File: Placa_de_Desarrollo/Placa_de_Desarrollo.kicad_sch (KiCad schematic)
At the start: 46 parts, among them J10 5V_OUT, J11 3.3V_OUT, J12 ADC_VREF, J13 GND, J14 AGND, J15 VSYS_ALIMEANTACION_EXTERNA, J16 3V3_EN, J17 DEVICE I2C0, J18 PINES GPIO, J19 ADC1, J2 USB_B_Micro, J20 ADC2, J21 ADC0, J3 DEVICE I2C0, J4 GND, J5 GND, J6 GND, J7 GND, J8 GND, J9 GND, SW1 RESET, U1 Pico, U2 LM317_TO-220

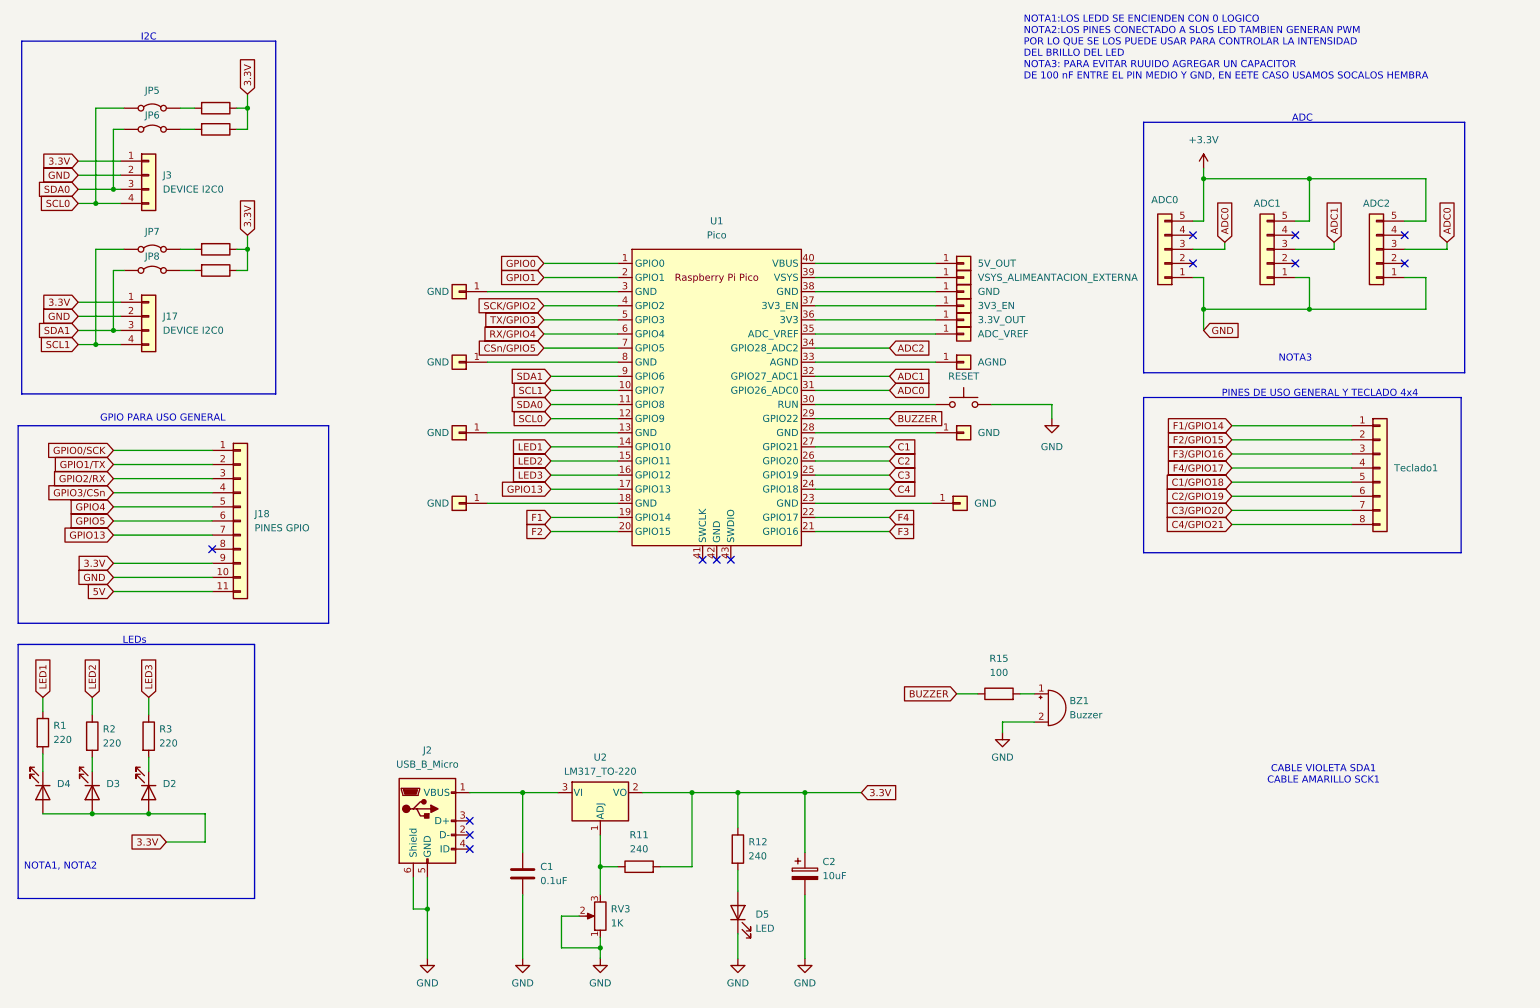
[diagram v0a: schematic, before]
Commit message: Actualizacion de placa de prueba
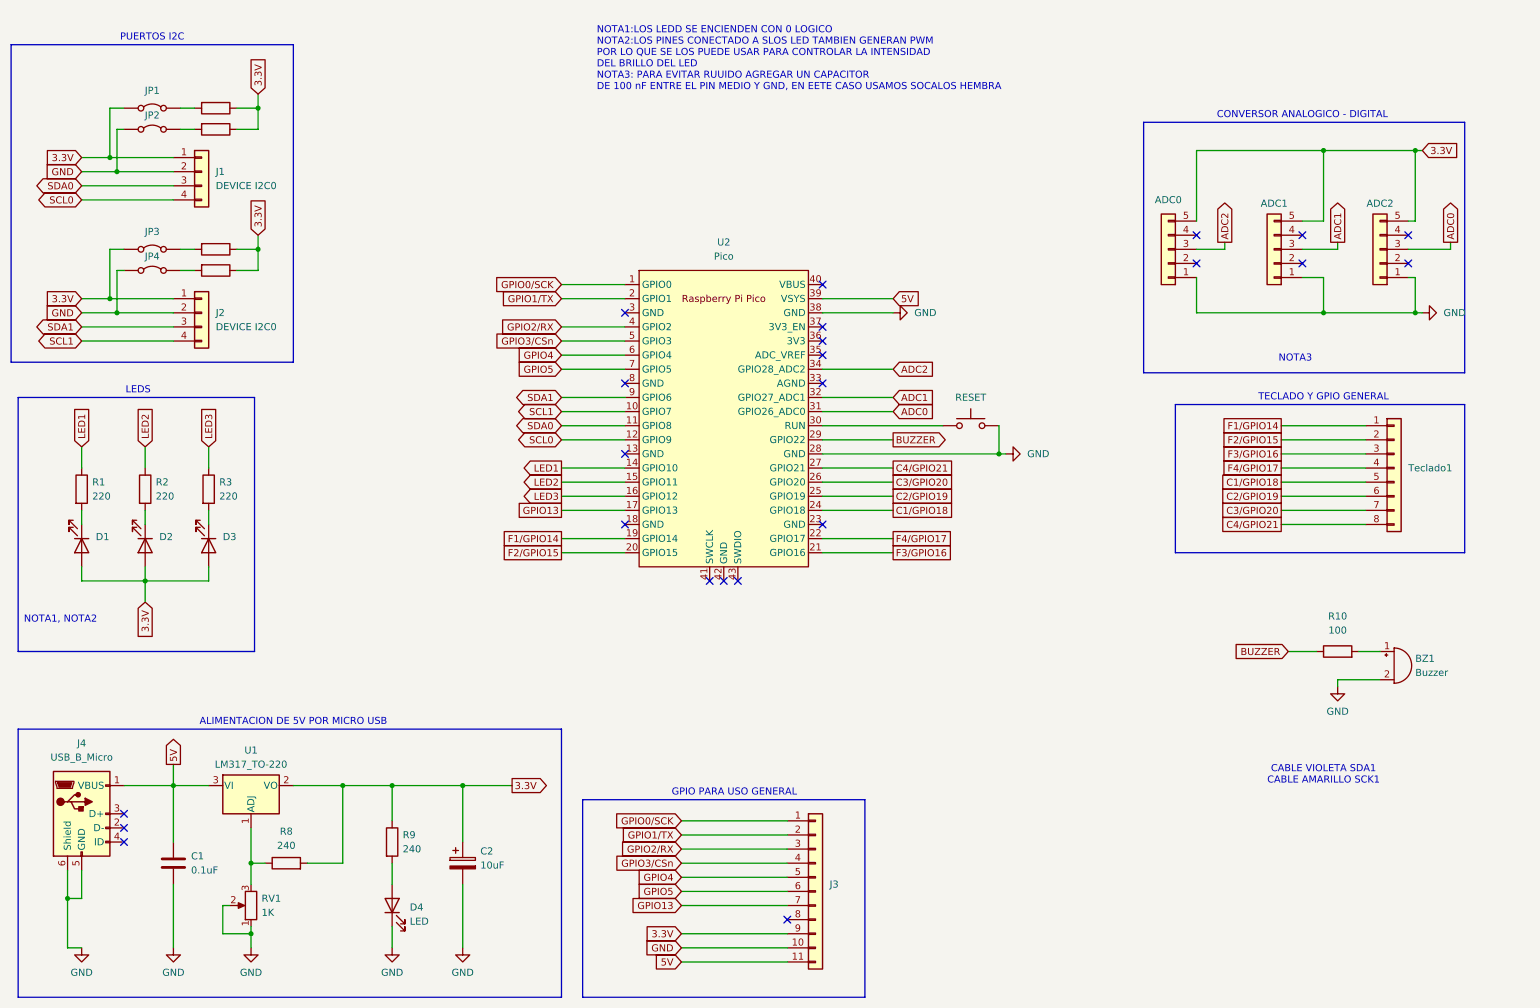
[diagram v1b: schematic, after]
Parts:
- removed J10: 5V_OUT, symbol Connector_Generic:Conn_01x01
- removed J11: 3.3V_OUT, symbol Connector_Generic:Conn_01x01
- removed J12: ADC_VREF, symbol Connector_Generic:Conn_01x01
- removed J13, J4, J5, J6, J7, J8, J9: GND, symbol Connector_Generic:Conn_01x01
- removed J14: AGND, symbol Connector_Generic:Conn_01x01
- removed J15: VSYS_ALIMEANTACION_EXTERNA, symbol Connector_Generic:Conn_01x01
- removed J16: 3V3_EN, symbol Connector_Generic:Conn_01x01
- renumbered D4 to D1, D3 to D2, D2 to D3, D5 to D4, J3 to J1, J21 to J18, J17 to J2, J18 to J3, J2 to J4, JP5 to JP1, JP6 to JP2, JP7 to JP3, JP8 to JP4, R15 to R10, R9 to R4, R10 to R5, R13 to R6, R14 to R7, R11 to R8, R12 to R9, RV3 to RV1, U2 to U1, U1 to U2
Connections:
- net +3.3V is gone; now on net 3.3V: J18.5 (Pin_5), J19.5 (Pin_5), J20.5 (Pin_5)
- net C1 is gone; now on net C4/GPIO21: U2.27 (GPIO21)
- net C2 is gone; now on net C3/GPIO20: U2.26 (GPIO20)
- net C3 is gone; now on net C2/GPIO19: U2.25 (GPIO19)
- net C4 is gone; now on net C1/GPIO18: U2.24 (GPIO18)
- net CSn/GPIO5 is gone; now on net GPIO5: U2.7 (GPIO5)
- net F1 is gone; now on net F1/GPIO14: U2.19 (GPIO14)
- net F2 is gone; now on net F2/GPIO15: U2.20 (GPIO15)
- net F3 is gone; now on net F3/GPIO16: U2.21 (GPIO16)
- net F4 is gone; now on net F4/GPIO17: U2.22 (GPIO17)
- net GPIO0 is gone; now on net GPIO0/SCK: U2.1 (GPIO0)
- net GPIO1 is gone; now on net GPIO1/TX: U2.2 (GPIO1)
- net RX/GPIO4 is gone; now on net GPIO4: U2.6 (GPIO4)
- net SCK/GPIO2 is gone; now on net GPIO2/RX: U2.4 (GPIO2)
- net TX/GPIO3 is gone; now on net GPIO3/CSn: U2.5 (GPIO3)
- net 3.3V: now also JP1.1 (A), JP3.1 (A)
- net 5V: now also C1.1, J4.1 (VBUS), U1.3 (VI), U2.39 (VSYS)
- net ADC0: no longer J18.3 (Pin_3)
- net ADC2: now also J18.3 (Pin_3)
- net GND: now also JP2.1 (A), JP4.1 (A), U2.28 (GND), U2.38 (GND)
- net SCL0: no longer JP1.1 (A)
- net SCL1: no longer JP3.1 (A)
- net SDA0: no longer JP2.1 (A)
- net SDA1: no longer JP4.1 (A)
- no-connect marks 13 -> 23
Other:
- note added: "ALIMENTACION DE 5V POR MICRO USB"
- note added: "CONVERSOR ANALOGICO - DIGITAL"
- note added: "LEDS"
- note added: "PUERTOS I2C"
- note added: "TECLADO Y GPIO GENERAL"
- note removed: "ADC"
- note removed: "I2C"
- note removed: "LEDs"
- note removed: "PINES DE USO GENERAL Y TECLADO 4x4"
- moved on the sheet: BZ1, C1, C2, D1, D2, D3, D4, J1, J2, J3, J4, R1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

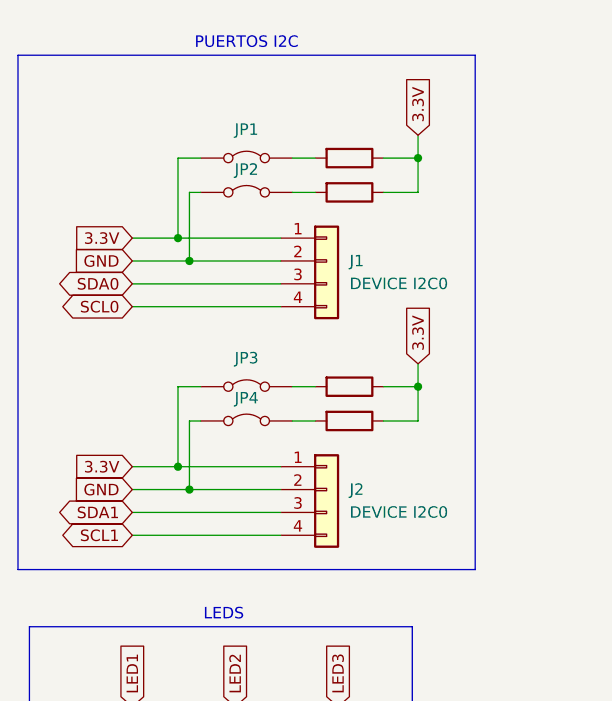
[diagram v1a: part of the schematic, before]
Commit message: Actualizacion de respo Kicad
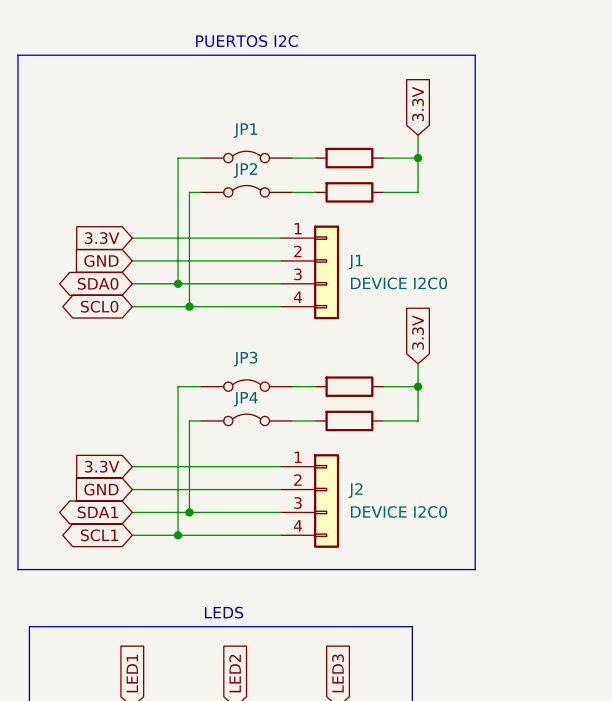
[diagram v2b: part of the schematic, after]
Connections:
- net 3.3V: no longer JP1.1 (A), JP3.1 (A)
- net GND: no longer JP2.1 (A), JP4.1 (A)
- net SCL0: now also JP2.1 (A)
- net SCL1: now also JP3.1 (A)
- net SDA0: now also JP1.1 (A)
- net SDA1: now also JP4.1 (A)
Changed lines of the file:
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@@
-	)
-	(junction
-		(at 34.29 41.91)
-		(diameter 0)
-		(color 0 0 0 0)
 	)
 	(junction
@@
 	)
 	(junction
+		(at 35.56 49.53)
+		(diameter 0)
+		(color 0 0 0 0)
+	)
+	(junction
 		(at 45.72 154.94)
 		(diameter 0)
@@
 	)
 	(junction
+		(at 34.29 46.99)
+		(diameter 0)
+		(color 0 0 0 0)
+	)
+	(junction
 		(at 60.96 33.02)
 		(diameter 0)
@@
 	)
 	(junction
-		(at 35.56 44.45)
-		(diameter 0)
-		(color 0 0 0 0)
-	)
-	(junction
 		(at 59.69 168.91)
 		(diameter 0)
@@
 	)
 	(junction
-		(at 35.56 69.85)
-		(diameter 0)
-		(color 0 0 0 0)
-	)
-	(junction
-		(at 34.29 67.31)
+		(at 34.29 74.93)
 		(diameter 0)
 		(color 0 0 0 0)
@@
 		(color 0 0 0 0)
 	)
+	(junction
+		(at 35.56 72.39)
+		(diameter 0)
+		(color 0 0 0 0)
+	)
 	(no_connect
 		(at 36.83 160.02)
@@
 	(wire
 		(pts
-			(xy 34.29 58.42) (xy 34.29 67.31)
-		)
-		(stroke
-			(width 0)
-			(type default)
-		)
-	)
-	(wire
-		(pts
 			(xy 162.56 100.33) (xy 175.26 100.33)
 		)
@@
 	(wire
 		(pts
+			(xy 34.29 58.42) (xy 34.29 74.93)
+		)
+		(stroke
+			(width 0)
+			(type default)
+		)
+	)
+	(wire
+		(pts
 			(xy 137.16 173.99) (xy 156.21 173.99)
 		)
@@
 	(wire
 		(pts
+			(xy 34.29 74.93) (xy 45.72 74.93)
+		)
+		(stroke
+			(width 0)
+			(type default)
+		)
+	)
+	(wire
+		(pts
 			(xy 267.97 63.5) (xy 269.24 63.5)
 		)
@@
 	(wire
 		(pts
-			(xy 29.21 41.91) (xy 34.29 41.91)
-		)
-		(stroke
-			(width 0)
-			(type default)
-		)
-	)
-	(wire
-		(pts
 			(xy 115.57 74.93) (xy 127 74.93)
 		)
@@
 	(wire
 		(pts
-			(xy 34.29 33.02) (xy 34.29 41.91)
-		)
-		(stroke
-			(width 0)
-			(type default)
-		)
-	)
-	(wire
-		(pts
 			(xy 248.92 63.5) (xy 252.73 63.5)
 		)
@@
 	(wire
 		(pts
-			(xy 29.21 49.53) (xy 45.72 49.53)
+			(xy 29.21 49.53) (xy 35.56 49.53)
 		)
 		(stroke
@@
 	(wire
 		(pts
-			(xy 29.21 44.45) (xy 35.56 44.45)
-		)
-		(stroke
-			(width 0)
-			(type default)
-		)
-	)
-	(wire
-		(pts
 			(xy 60.96 36.83) (xy 60.96 33.02)
 		)
@@
 	(wire
 		(pts
-			(xy 35.56 36.83) (xy 35.56 44.45)
-		)
-		(stroke
-			(width 0)
-			(type default)
-		)
-	)
-	(wire
-		(pts
 			(xy 275.59 58.42) (xy 267.97 58.42)
 		)
@@
 	(wire
 		(pts
+			(xy 35.56 72.39) (xy 45.72 72.39)
+		)
+		(stroke
+			(width 0)
+			(type default)
+		)
+	)
+	(wire
+		(pts
 			(xy 275.59 57.15) (xy 275.59 58.42)
 		)
@@
 	(wire
 		(pts
-			(xy 29.21 69.85) (xy 35.56 69.85)
-		)
-		(stroke
-			(width 0)
-			(type default)
-		)
-	)
-	(wire
-		(pts
 			(xy 76.2 168.91) (xy 76.2 154.94)
 		)
@@
 	(wire
 		(pts
-			(xy 34.29 41.91) (xy 45.72 41.91)
+			(xy 29.21 41.91) (xy 45.72 41.91)
 		)
 		(stroke
@@
 	(wire
 		(pts
+			(xy 35.56 36.83) (xy 35.56 49.53)
+		)
+		(stroke
+			(width 0)
+			(type default)
+		)
+	)
+	(wire
+		(pts
 			(xy 52.07 115.57) (xy 52.07 118.11)
 		)
@@
 	(wire
 		(pts
-			(xy 35.56 69.85) (xy 45.72 69.85)
+			(xy 29.21 69.85) (xy 45.72 69.85)
 		)
 		(stroke
@@
 	(wire
 		(pts
+			(xy 34.29 46.99) (xy 45.72 46.99)
+		)
+		(stroke
+			(width 0)
+			(type default)
+		)
+	)
+	(wire
+		(pts
 			(xy 46.99 58.42) (xy 49.53 58.42)
 		)
@@
 	(wire
 		(pts
+			(xy 35.56 62.23) (xy 35.56 72.39)
+		)
+		(stroke
+			(width 0)
+			(type default)
+		)
+	)
+	(wire
+		(pts
 			(xy 252.73 63.5) (xy 252.73 69.85)
 		)
@@
 	(wire
 		(pts
+			(xy 34.29 33.02) (xy 34.29 46.99)
+		)
+		(stroke
+			(width 0)
+			(type default)
+		)
+	)
+	(wire
+		(pts
 			(xy 97.79 154.94) (xy 85.09 154.94)
 		)
@@
 	(wire
 		(pts
+			(xy 35.56 49.53) (xy 45.72 49.53)
+		)
+		(stroke
+			(width 0)
+			(type default)
+		)
+	)
+	(wire
+		(pts
 			(xy 115.57 67.31) (xy 127 67.31)
 		)
@@
 	(wire
 		(pts
-			(xy 29.21 67.31) (xy 34.29 67.31)
+			(xy 29.21 67.31) (xy 45.72 67.31)
 		)
 		(stroke
@@
 	(wire
 		(pts
-			(xy 29.21 74.93) (xy 45.72 74.93)
-		)
-		(stroke
-			(width 0)
-			(type default)
-		)
-	)
-	(wire
-		(pts
-			(xy 35.56 62.23) (xy 35.56 69.85)
+			(xy 29.21 74.93) (xy 34.29 74.93)
 		)
 		(stroke
@@
 	(wire
 		(pts
-			(xy 34.29 67.31) (xy 45.72 67.31)
-		)
-		(stroke
-			(width 0)
-			(type default)
-		)
-	)
-	(wire
-		(pts
 			(xy 52.07 105.41) (xy 52.07 107.95)
 		)
@@
 	(wire
 		(pts
-			(xy 29.21 72.39) (xy 45.72 72.39)
+			(xy 29.21 72.39) (xy 35.56 72.39)
 		)
 		(stroke
@@
 	(wire
 		(pts
-			(xy 29.21 46.99) (xy 45.72 46.99)
+			(xy 29.21 46.99) (xy 34.29 46.99)
 		)
 		(stroke
@@
 	(wire
 		(pts
-			(xy 35.56 44.45) (xy 45.72 44.45)
-		)
-		(stroke
+			(xy 29.21 44.45) (xy 45.72 44.45)
+		)
+		(stroke
